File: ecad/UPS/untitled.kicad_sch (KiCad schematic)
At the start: 10 parts, among them U1 BQ25731RSNR

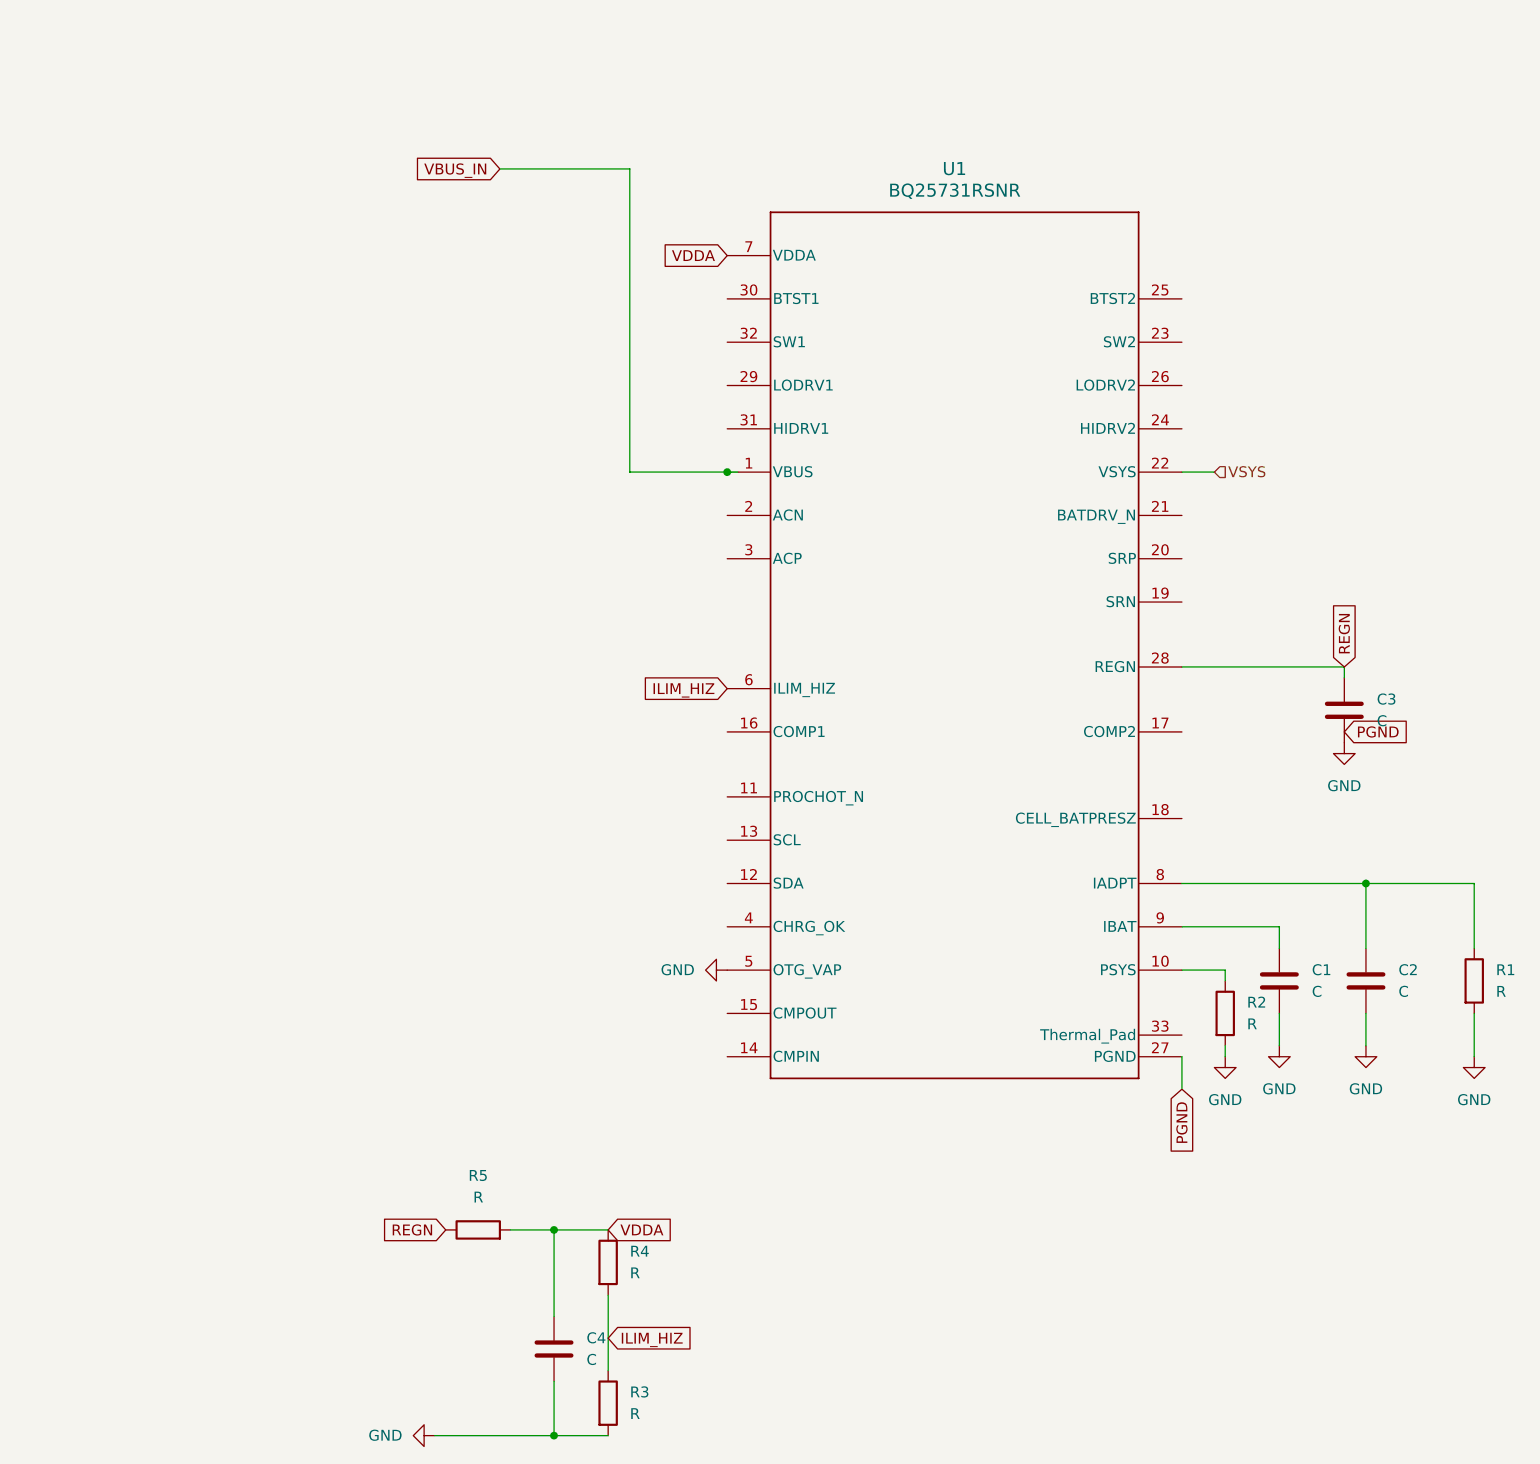
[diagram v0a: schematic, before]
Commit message: First half of BQ schematic
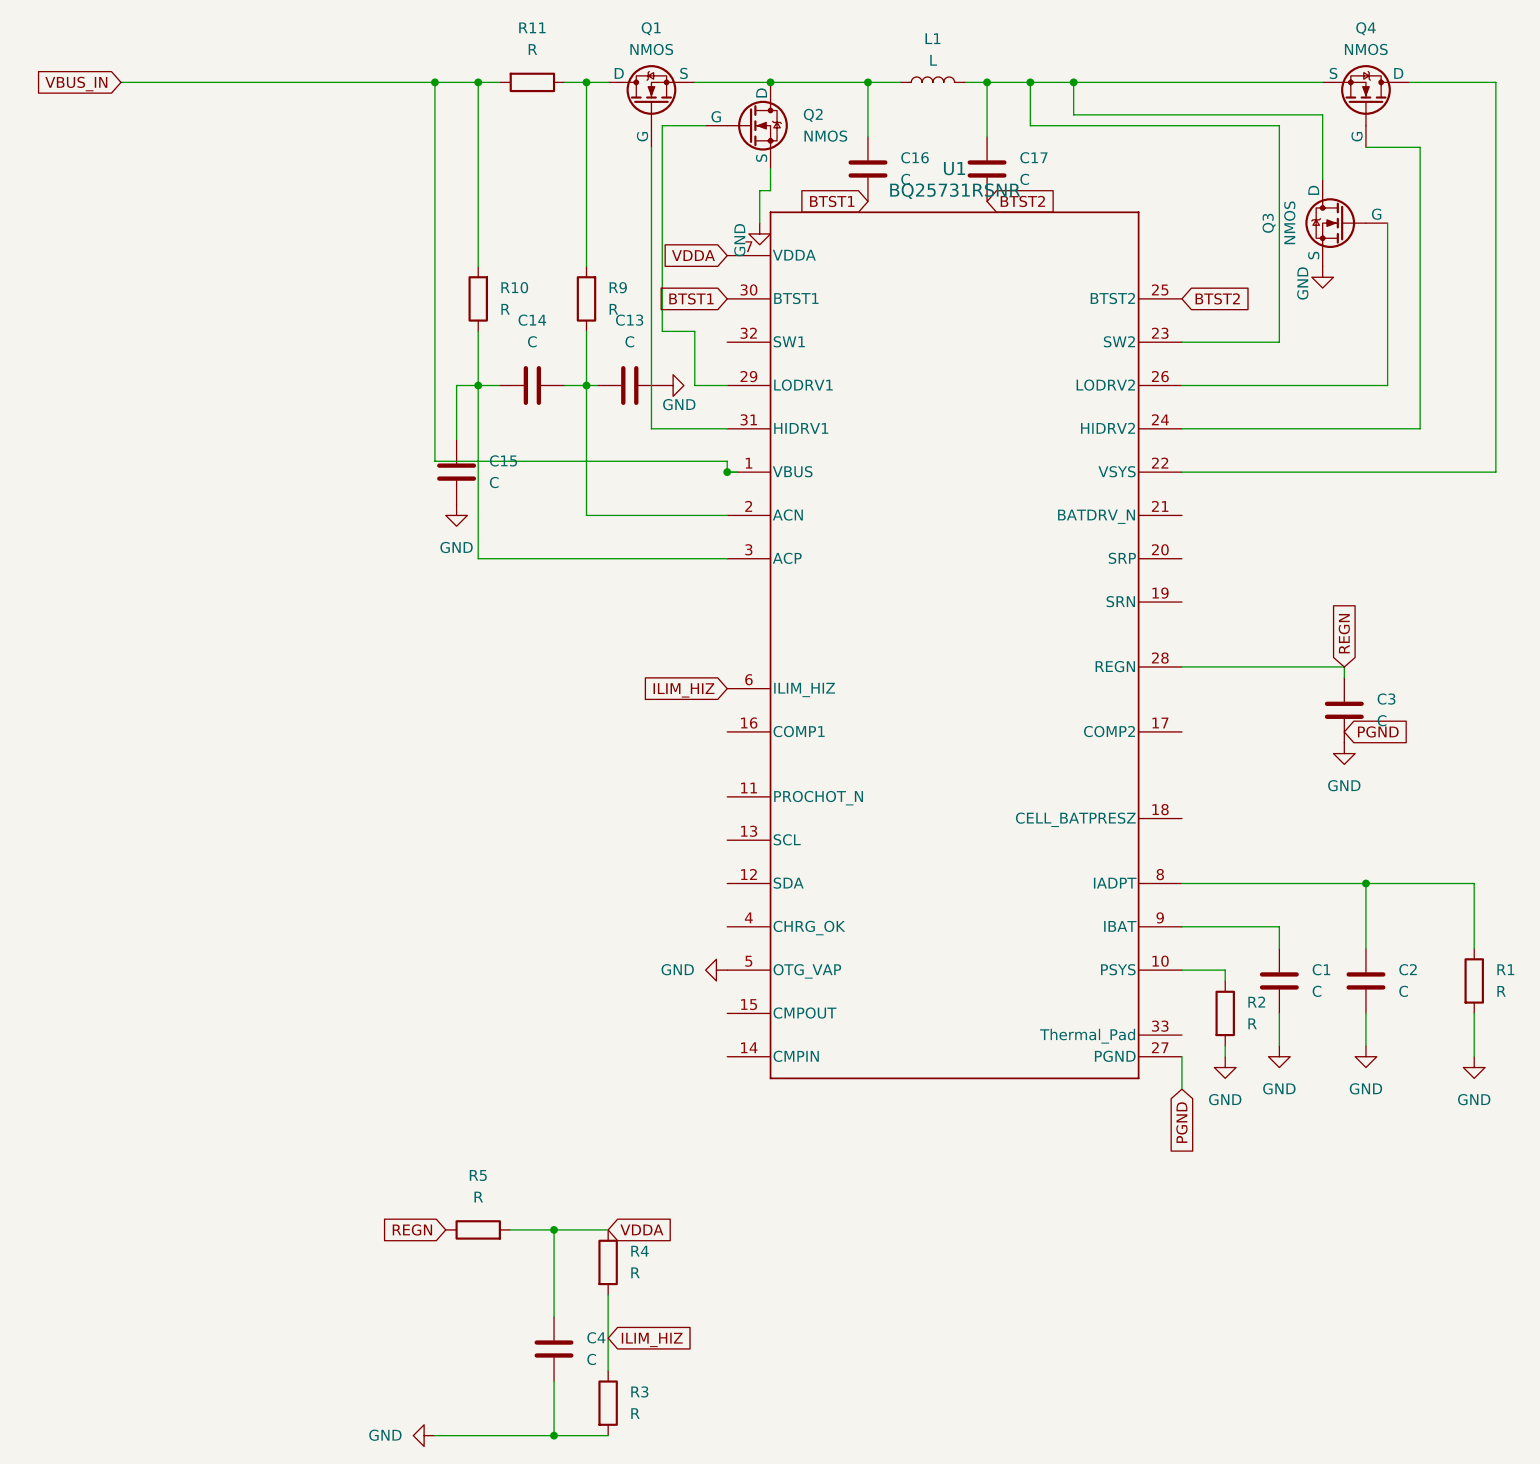
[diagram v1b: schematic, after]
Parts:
- added C13, C14, C15, C16, C17: C, symbol Device:C
- added L1: L, symbol Device:L
- added Q1, Q2, Q3, Q4: NMOS, symbol Simulation_SPICE:NMOS
- added R10, R11, R9: R, symbol Device:R
- U1: footprint UPS:RSN0032B-IPC_A -> RSN0032B-IPC_A
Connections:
- net GND: now also C13.2, C15.1, Q2.3 (S), Q3.3 (S)
- net VBUS_IN: now also R10.2, R11.2
- net at U1.2 (ACN): now also C13.1, C14.2, R9.1
- net at U1.23 (SW2): now also C17.2, L1.2, Q3.1 (D), Q4.3 (S)
- net at U1.24 (HIDRV2): now also Q4.2 (G)
- net BTST2: now reaches U1.25 (BTST2)
- net BTST2: now also C17.1
- net at U1.26 (LODRV2): now also Q3.2 (G)
- net at U1.29 (LODRV1): now also Q2.2 (G)
- net at U1.3 (ACP): now also C14.1, C15.2, R10.1
- net BTST1: now reaches U1.30 (BTST1)
- net BTST1: now also C16.1
- net at U1.31 (HIDRV1): now also Q1.2 (G)
- net VSYS: no longer names the net of U1.22 (VSYS)
- net VSYS: now also Q4.1 (D)
- new net: C16.2, L1.1, Q1.3 (S), Q2.1 (D)
- new net: Q1.1 (D), R11.1, R9.2
